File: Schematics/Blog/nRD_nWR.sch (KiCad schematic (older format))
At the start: 3 parts, among them U1 74HC04, U2 74HC32, U3 74HC08

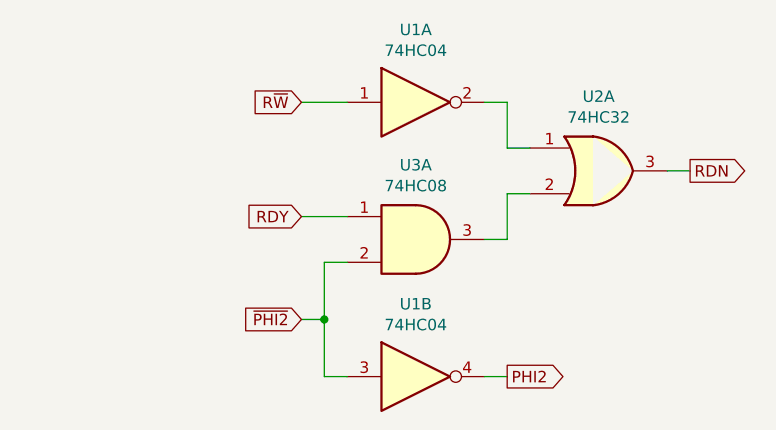
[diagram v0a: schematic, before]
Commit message: Updated Blog schematic
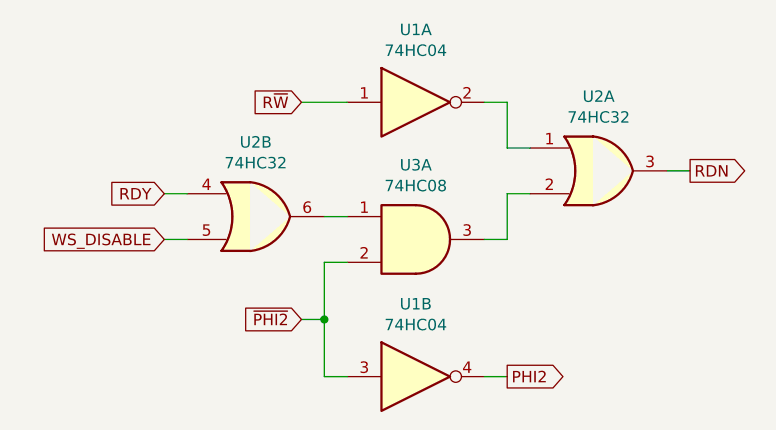
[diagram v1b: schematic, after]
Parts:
- added unit 2 of U2
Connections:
- net RDY: now also U2.4; no longer U3.1
- new net: U2.6, U3.1
- new net WS_DISABLE: U2.5
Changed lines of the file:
@@
 Wire Wire Line
 	3150 3250 3250 3250
-Text GLabel 2350 2550 0    50   Input ~ 0
+Text GLabel 1750 2450 0    50   Input ~ 0
 RDY
 Wire Wire Line
-	2350 2550 2550 2550
+	2450 2550 2550 2550
 Wire Wire Line
 	3150 2650 3250 2650
@@
 Text GLabel 3250 3250 2    50   Output ~ 0
 PHI2
+$Comp
+L 74xx:74LS32 U?
+U 2 1 60C815BD
+P 2150 2550
+AR Path="/60C815BD" Ref="U?"  Part="1"
+AR Path="/60B96DC5/60C815BD" Ref="U2"  Part="2"
+F 0 "U2" H 2150 2875 50  0000 C CNN
+F 1 "74HC32" H 2150 2784 50  0000 C CNN
+F 2 "" H 2150 2550 50  0001 C CNN
+F 3 "http://www.ti.com/lit/gpn/sn74LS32" H 2150 2550 50  0001 C CNN
+	2    2150 2550
+	1    0    0    -1
+$EndComp
+Wire Wire Line
+	1750 2450 1850 2450
+Text GLabel 1750 2650 0    50   Input ~ 0
+WS_DISABLE
+Wire Wire Line
+	1750 2650 1850 2650
 $EndSCHEMATC
